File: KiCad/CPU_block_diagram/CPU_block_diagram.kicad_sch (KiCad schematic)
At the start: 2 parts, among them SW1 SW_Push, SW2 SW_SPDT

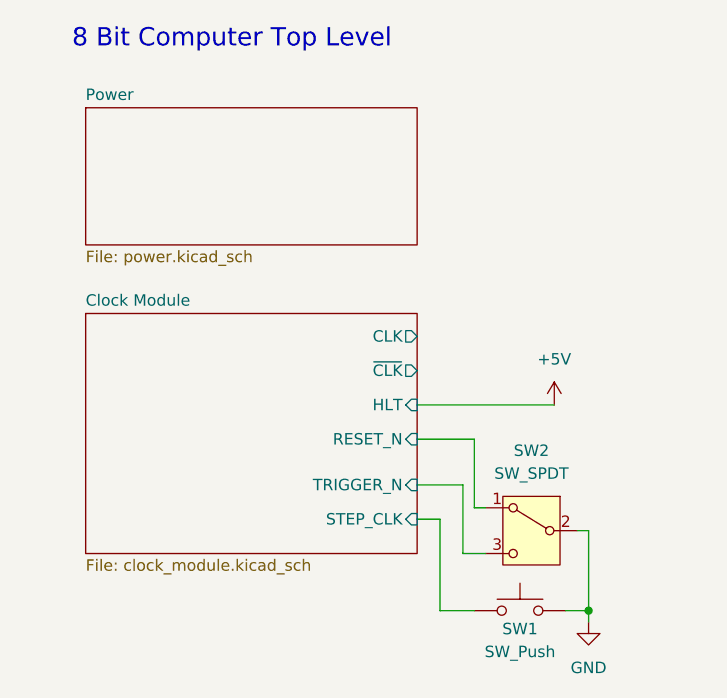
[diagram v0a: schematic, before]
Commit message: vault backup: 2025-12-30 22:01:07
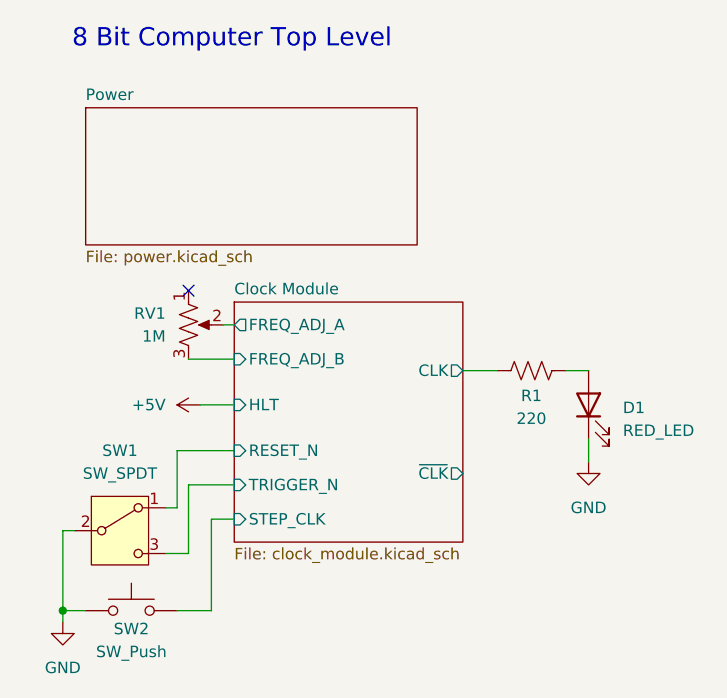
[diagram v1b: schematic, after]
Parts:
- added D1: RED_LED, symbol Device:LED
- added R1: 220, symbol Device:R_US
- added RV1: 1M, symbol Device:R_Potentiometer_US
- renumbered SW2 to SW1, SW1 to SW2
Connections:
- net Clock Module/CLK: now also R1.2
- net GND: now also D1.1 (K)
- new net: D1.2 (A), R1.1
- new net Clock Module/FREQ_ADJ_A: RV1.2
- new net Clock Module/FREQ_ADJ_B: RV1.3
- no-connect marks 0 -> 1
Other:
- sheet Clock Module ports: added FREQ_ADJ_A, FREQ_ADJ_B; removed none
- moved on the sheet: SW1, SW2
